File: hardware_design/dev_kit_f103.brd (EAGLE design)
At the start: 160 x 100 mm, 50 parts, among them U2 FT232RLSSOP, U7 AMS1117-3.3, Y1 32.768kHz

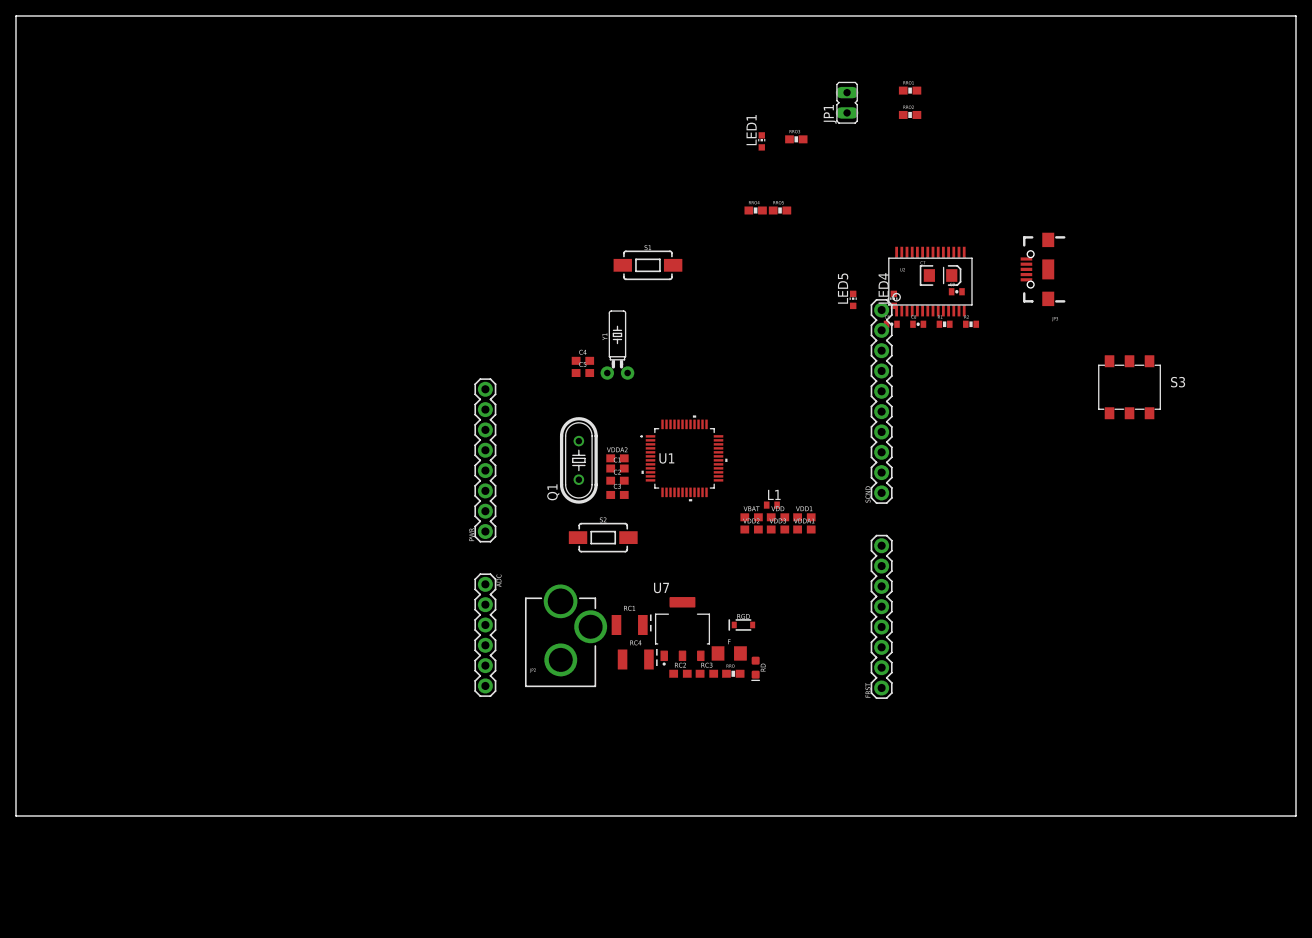
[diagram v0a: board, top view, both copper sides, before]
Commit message: Version 2 was started to design
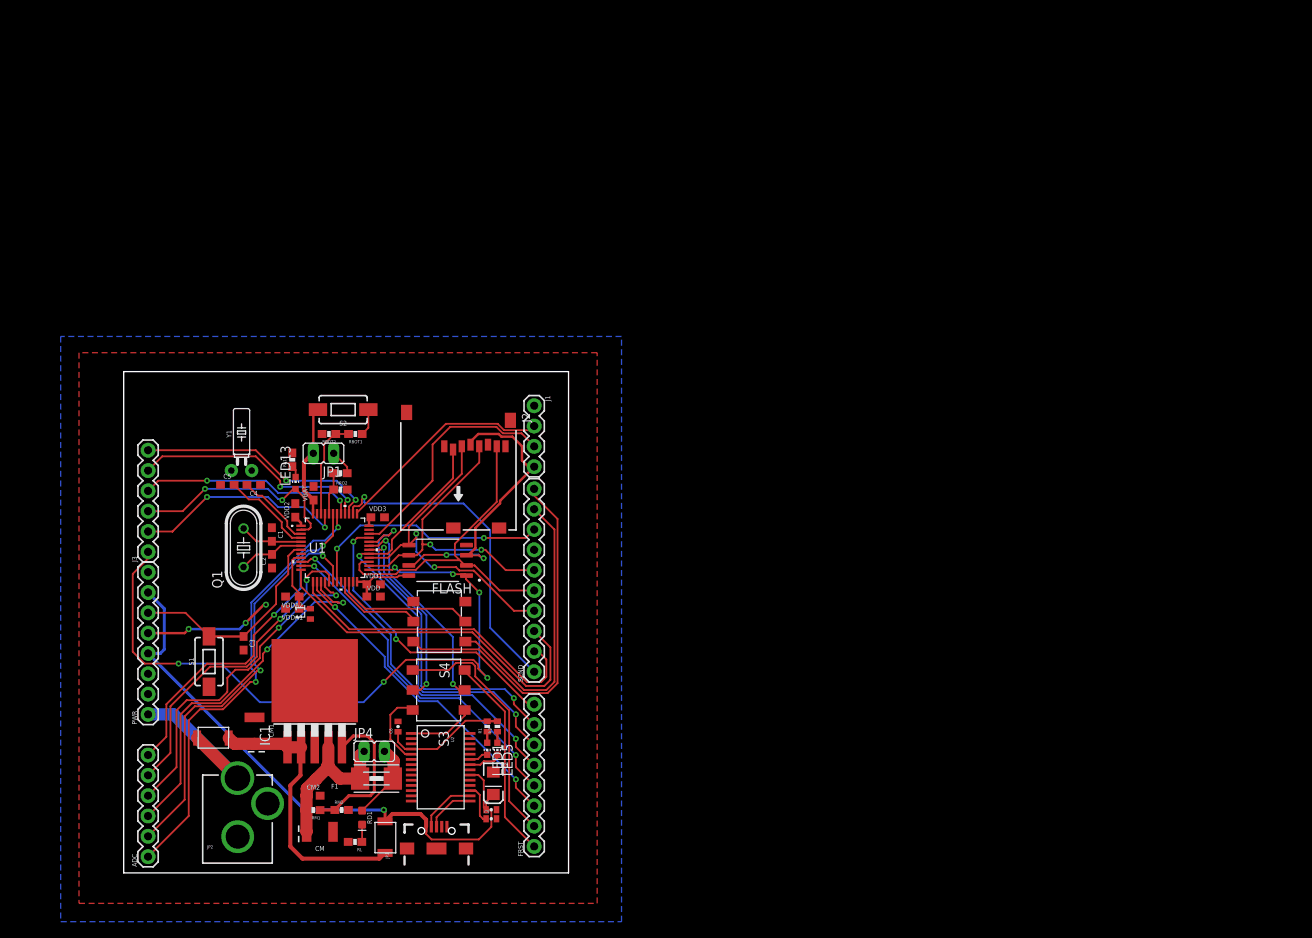
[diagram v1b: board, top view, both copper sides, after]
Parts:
- removed F: 0.75A, SparkFun-Fuses:1206
- removed LED4: (no value), adafruit:CHIP-LED0603
- removed RC1, RC4: 22uF, SparkFun-Capacitors:EIA3528
- removed RC2, RC3: 100nF, SparkFun-Capacitors:0603
- removed RD: Red, SparkFun-LED:LED-0603
- removed RGD: 1A/23V, SparkFun-DiscreteSemi:SOD-323
- removed RRO: 1.5k, SparkFun-Resistors:0603-RES
- removed RRO3: 470, SparkFun-Resistors:0603-RES
- removed RRO4: 10k, SparkFun-Resistors:0603-RES
- removed RRO5: 330, SparkFun-Resistors:0603-RES
- removed U7: AMS1117-3.3, AMS1117-3.3:SOT229P700X180-4N
- added CM, CM1: 10uF, SparkFun-Capacitors:EIA3528
- added CM2: 100nF, SparkFun-Capacitors:0603
- added D1, D2: (no value), 1N4007:3ASCHOOTKY
- added F1: (no value), adafruit:1812
- added FLASH: (no value), W25Q64:W25Q64
- added IC1: (no value), MIC29302WU:TO263-5
- added J1: (no value), SparkFun-Connectors:1X04
- added J2: CON-SD-CARD_MICROSD-2908-05, 52101-101-REV-A_v16:CON-SD-CARD_2908-05
- added J3: (no value), SparkFun-Connectors:1X06
- added JP4: (no value), jumper:JP1
- added LED13: (no value), adafruit:CHIP-LED0603
- added RBOT1: 330, SparkFun-Resistors:0603-RES
- added RBOT2: 10k, SparkFun-Resistors:0603-RES
- added RD1: Red, SparkFun-LED:LED-0603
- added RL: 1.5k, SparkFun-Resistors:0603-RES
- added RL13: 470, SparkFun-Resistors:0603-RES
- added RM1: 316, SparkFun-Resistors:0603-RES
- added RM2: 187, SparkFun-Resistors:0603-RES
- added S4: (no value), step_switch:452403012014
- moved JP3 105.3 mm to (52.6, -4.06), turned to 90 degrees
- moved S3 94.3 mm to (52.8, 15.7), turned to 270 degrees
- moved C9 87.9 mm to (59.4, -0.35)
- moved RRO1 86.9 mm to (40.6, 40.8)
- moved U2 86.2 mm to (53.1, 6.10), turned to 270 degrees
- moved C7 84.6 mm to (59.7, 4.09), turned to 270 degrees
- moved RRO2 84.1 mm to (40.5, 42.8), turned to 180 degrees
- moved LED1 83.3 mm to (58.9, 8.41), turned to 180 degrees
- moved C8 82.2 mm to (47.8, 11.2), turned to 90 degrees
- moved JP1 78.8 mm to (38.4, 45.3), turned to 90 degrees
- moved C6 78.7 mm to (59.4, 0.79)
- moved R2 77.7 mm to (60.2, 11.2), turned to 90 degrees
- moved R1 76.1 mm to (58.9, 11.2), turned to 90 degrees
- moved S1 73.9 mm to (24.1, 19.3), turned to 90 degrees
- moved LED5 71.6 mm to (60.2, 8.41), turned to 180 degrees
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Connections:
- removed net MISO1: U1.16
- removed net MOSI1: U1.17
- removed net N$10: U1.19
- removed net N$11: U1.25
- removed net N$12: U1.26
- removed net N$13: U1.27
- removed net N$14: U1.28
- removed net N$15: U1.39
- removed net N$16: U1.40
- removed net N$17: U1.41
- removed net N$18: U1.45
- removed net N$19: U1.46
- removed net N$21: U1.11
- removed net N$22: U1.14
- removed net N$23: U1.29
- removed net N$24: U1.32
- removed net N$25: U1.33
- removed net N$26: U1.34
- removed net N$27: U1.37
- removed net N$28: U1.38
- removed net N$29: FRST.8
- removed net N$30: FRST.7
- removed net N$31: FRST.6
- removed net N$32: FRST.5
- removed net N$33: FRST.4
- removed net N$34: FRST.3
- removed net N$9: U1.18
- removed net SCK1: U1.15
- new net CRX3: S4.1
- new net CS2: FLASH.CS, J3.1, U1.25
- new net CSCL: S4.6, SCND.10
- new net CSDA: S4.3, SCND.9
- new net CTX3: S4.4
- new net MISO2: FLASH.DO, J2.7, SCND.5, U1.27
- new net MOSI2: FLASH.DI, J2.3, SCND.4, U1.28
- new net N$35: RD1.C, RL.1
- new net PA11: FRST.7, U1.32
- new net PA12: FRST.8, U1.33
- new net PA15: SCND.1, U1.38
- new net PA4: FRST.3, U1.14
- new net PA5: ADC.3, U1.15
- new net PA6: ADC.4, U1.16
- new net PA7: ADC.5, U1.17
- new net PA8: FRST.6, J2.2, U1.29
- new net PB3: J3.6, U1.39
- new net PB4: J3.5, U1.40
- new net PB5: J3.4, U1.41
- new net PB8: J3.2, U1.45
- new net SCK2: FLASH.CLK, J2.5, SCND.6, U1.26
- new net SWCLK: J1.2, U1.37
- new net SWDIO: J1.3, U1.34
- net 3.3V: now also F1.2, FLASH.H/R, FLASH.VCC, FLASH.WP, J1.4, J2.4, JP4.2, PWR.5, RD1.A; no longer F.2, RD.A
- net BUTTON: now also RBOT1.2, RBOT2.1, U1.46; no longer RRO4.1, RRO5.2
- net GND: now also CM.C, CM1.C, CM2.2, FLASH.GND, IC1.3, IC1.6, J1.1, J2.6, PWR.2, PWR.3, RBOT2.2, RL.2, RL13.2, RM2.2, SCND.7; no longer RC1.C, RC2.2, RC3.2, RC4.C, RRO.2, RRO3.2, RRO4.2, U7.1
- net LED: now also J3.3, LED13.A; no longer LED4.A
- net N$1: now also CM1.A, D1.OUT, D2.OUT, IC1.1, IC1.2; no longer F.1, RC3.1, RC4.A, U7.2
- net N$2: now also CM.A, CM2.1, F1.1, IC1.4, JP4.1, RM1.2; no longer RD.C, RRO.1
- net N$20: now also IC1.5, RM1.1, RM2.1; no longer U1.10
- net N$4: now also LED13.C, RL13.1; no longer LED4.C, RRO3.1
- net N$5: now also RBOT1.1; no longer RRO5.1
- net NRST: now also PWR.6
- net PA0: now also FRST.5, U1.10; no longer ADC.6
- net PA1: now also FRST.4, U1.11; no longer ADC.5
- net PB0: now also ADC.6, U1.18; no longer ADC.4
- net PB1: now also SCND.8, U1.19; no longer ADC.3
- net RX2: now also SCND.2
- net RX3/SDA2: now also S4.2
- net TX2: now also SCND.3
- net TX3/SCL2: now also S4.5
- net VIN: now also D2.IN, PWR.1; no longer RC1.A, RC2.1, RGD.C, U7.3
- net V_USB: now also D1.IN, PWR.4, PWR.7; no longer RGD.A
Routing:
- net CS2: track 0.00 -> 90.3 mm, vias 0 -> 6
- net 3.3V: track 0.00 -> 89.9 mm, vias 0 -> 5
- net V_USB: track 0.00 -> 76.7 mm, vias 0 -> 1
- net PA8: track 0.00 -> 57.9 mm, vias 0 -> 2
- net SCL1: track 0.00 -> 56.2 mm, vias 0 -> 2
- net SDA1: track 0.00 -> 53.5 mm, vias 0 -> 2
- net CSCL: track 0.00 -> 46.7 mm
- net TX2: track 0.00 -> 45.7 mm
- net PA5: track 0.00 -> 45.5 mm, vias 0 -> 2
- net MISO2: track 0.00 -> 43.7 mm
- net PA1: track 0.00 -> 43.3 mm, vias 0 -> 2
- net PA11: track 0.00 -> 43.0 mm, vias 0 -> 2
- net PA0: track 0.00 -> 42.7 mm, vias 0 -> 2
- net MOSI2: track 0.00 -> 42.6 mm, vias 0 -> 2
- net PA6: track 0.00 -> 42.4 mm, vias 0 -> 2
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- added copper zone on layer 1, net GND
- added copper zone on layer 16, net GND
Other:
- board size 160 x 100 mm -> 55.6 x 62.7 mm
